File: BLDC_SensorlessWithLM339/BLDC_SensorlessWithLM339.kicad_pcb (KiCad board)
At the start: 2 copper layers, 98 x 98 mm, 48 parts, among them J1 Conn_01x04_Female, J2 Conn_01x07_Female, J3 Screw_Terminal_01x02, J4 Screw_Terminal_01x03, Q1 50N06, Q2 50N06, Q3 50N06, Q4 50N06, Q5 50N06, Q6 50N06, U1 IR2101, U2 IR2101, U3 IR2101, U4 LM339N

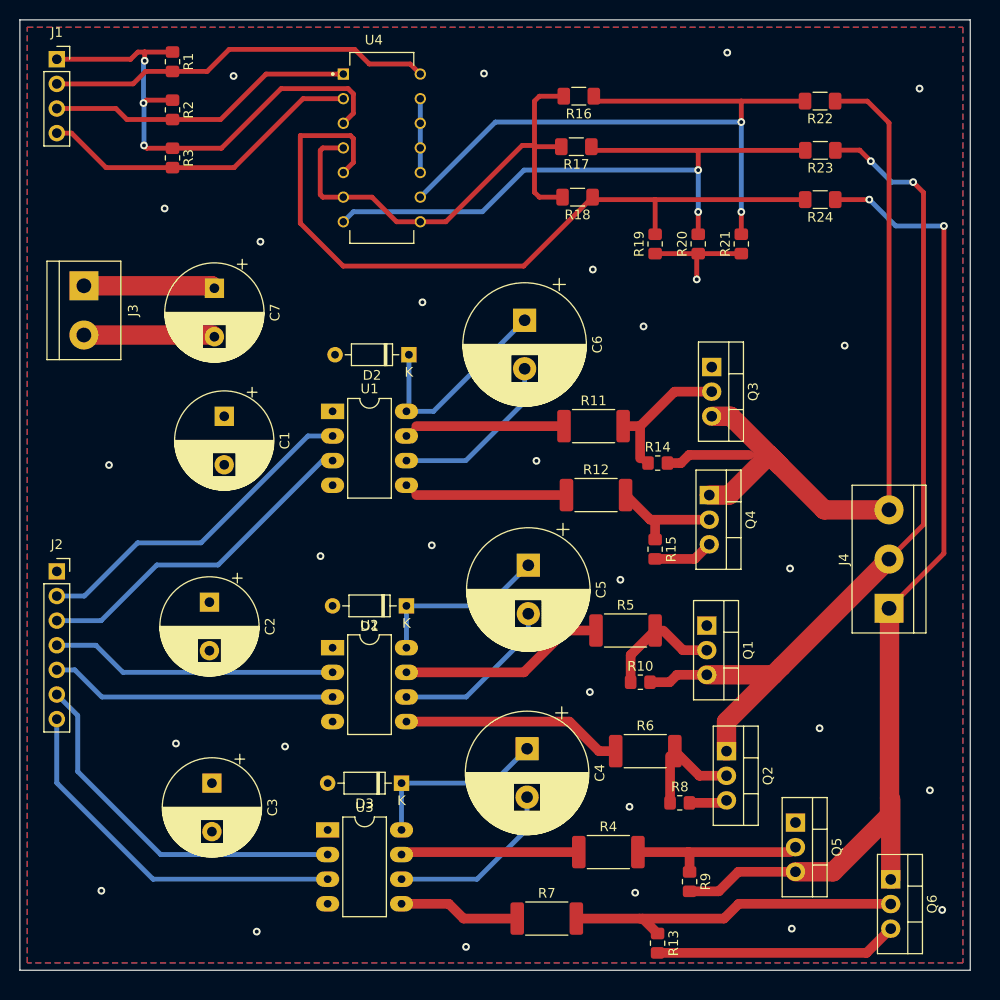
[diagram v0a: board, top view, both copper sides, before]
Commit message: Version 0.3
I ordered the PCB. I will test it when it arrives.
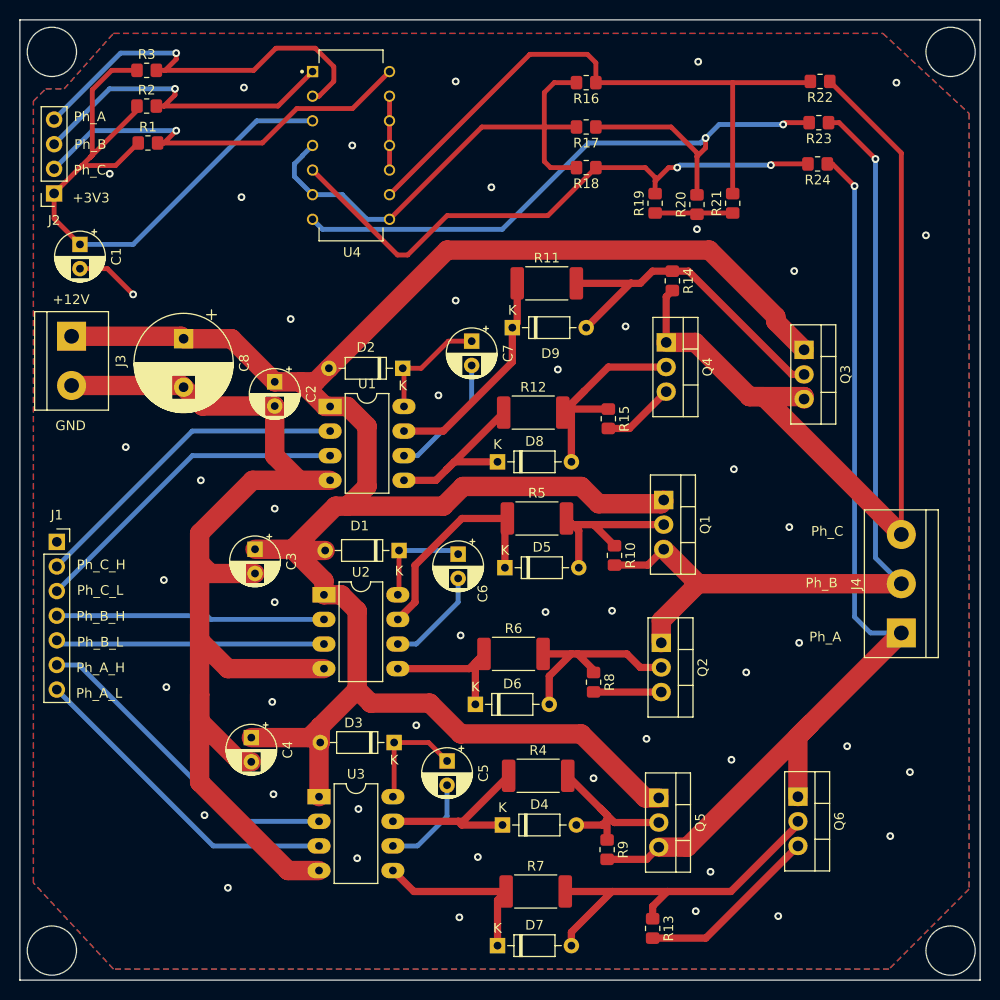
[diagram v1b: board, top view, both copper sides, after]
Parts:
- added C8: 470u, Capacitor_THT:CP_Radial_D10.0mm_P5.00mm, F.Cu at (28.8, 44.8)
- added D4: 1N4148, Diode_THT:D_DO-35_SOD27_P7.62mm_Horizontal, F.Cu at (61.7, 95.0)
- added D5: 1N4148, Diode_THT:D_DO-35_SOD27_P7.62mm_Horizontal, F.Cu at (62.0, 68.5)
- added D6: 1N4148, Diode_THT:D_DO-35_SOD27_P7.62mm_Horizontal, F.Cu at (58.9, 82.5)
- added D7: 1N4148, Diode_THT:D_DO-35_SOD27_P7.62mm_Horizontal, F.Cu at (61.2, 107.4)
- added D8: 1N4148, Diode_THT:D_DO-35_SOD27_P7.62mm_Horizontal, F.Cu at (61.2, 57.5)
- added D9: 1N4148, Diode_THT:D_DO-35_SOD27_P7.62mm_Horizontal, F.Cu at (62.7, 43.7)
- C1, C2, C3: footprint Capacitor_THT:CP_Radial_D10.0mm_P5.00mm -> Capacitor_THT:CP_Radial_D5.0mm_P2.50mm
- C4: value 2u2 -> 10u; footprint Capacitor_THT:CP_Radial_D12.5mm_P5.00mm -> Capacitor_THT:CP_Radial_D5.0mm_P2.50mm
- C5, C6: footprint Capacitor_THT:CP_Radial_D12.5mm_P5.00mm -> Capacitor_THT:CP_Radial_D5.0mm_P2.50mm
- C7: value 470u -> 2u2; footprint Capacitor_THT:CP_Radial_D10.0mm_P5.00mm -> Capacitor_THT:CP_Radial_D5.0mm_P2.50mm
- J1: value Conn_01x04_Female -> Conn_01x07_Female; footprint Connector_PinSocket_2.54mm:PinSocket_1x04_P2.54mm_Vertical -> Connector_PinSocket_2.54mm:PinSocket_1x07_P2.54mm_Vertical
- J2: value Conn_01x07_Female -> Conn_01x04_Female; footprint Connector_PinSocket_2.54mm:PinSocket_1x07_P2.54mm_Vertical -> Connector_PinSocket_2.54mm:PinSocket_1x04_P2.54mm_Vertical
- R10, R13, R14, R15, R8, R9: value 220 -> 10k
- R11, R12, R4, R5, R6, R7: value 10_2W -> 10_1W
- R16, R17, R18, R22, R23, R24: footprint Resistor_SMD:R_1206_3216Metric_Pad1.30x1.75mm_HandSolder -> Resistor_SMD:R_0805_2012Metric_Pad1.20x1.40mm_HandSolder
- moved J1 49.8 mm to (15.7, 65.8)
- moved J2 39.0 mm to (15.5, 29.8), turned to 180 degrees
- moved C4 28.5 mm to (35.8, 86.0)
- moved C7 27.1 mm to (58.5, 45.1)
- moved C6 25.1 mm to (57.1, 67.1)
- moved C3 24.5 mm to (36.2, 66.5)
- moved C2 23.7 mm to (38.2, 49.3)
- moved C1 23.1 mm to (18.1, 35.1)
- moved C5 21.9 mm to (56.0, 88.4)
- moved R14 18.9 mm to (79.2, 38.9), turned to 270 degrees
- moved R6 16.9 mm to (62.9, 77.3)
- moved Q4 16.4 mm to (78.6, 45.2)
- moved R11 15.5 mm to (66.3, 39.1)
- moved R8 15.3 mm to (71.1, 80.3), turned to 270 degrees
- moved R5 14.7 mm to (65.3, 63.4)
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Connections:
- C1 pad 1: +12V -> +3V3
- C4 pad 1: Net-(C4-Pad1) -> +12V
- C4 pad 2: Net-(C4-Pad2) -> GND
- C7 pad 1: +12V -> Net-(C7-Pad1)
- C7 pad 2: GND -> Net-(C7-Pad2)
- D1 pad 1: Net-(C5-Pad1) -> Net-(C6-Pad1)
- D2 pad 1: Net-(C6-Pad1) -> Net-(C7-Pad1)
- D3 pad 1: Net-(C4-Pad1) -> Net-(C5-Pad1)
- J1 pad 1: +3V3 -> Net-(J1-Pad1)
- J2 pad 1: Net-(J2-Pad1) -> +3V3
- R1 pad 2: Net-(J1-Pad2) -> Net-(J2-Pad2)
- R2 pad 2: Net-(J1-Pad3) -> Net-(J2-Pad3)
- R3 pad 2: Net-(J1-Pad4) -> Net-(J2-Pad4)
- U1 pad 2: Net-(J2-Pad2) -> Net-(J1-Pad2)
- U1 pad 3: Net-(J2-Pad3) -> Net-(J1-Pad3)
- U1 pad 6: Net-(C6-Pad2) -> Net-(C7-Pad2)
- U1 pad 8: Net-(C6-Pad1) -> Net-(C7-Pad1)
- U2 pad 2: Net-(J2-Pad4) -> Net-(J1-Pad4)
- U2 pad 3: Net-(J2-Pad5) -> Net-(J1-Pad5)
- U2 pad 6: Net-(C5-Pad2) -> Net-(C6-Pad2)
- U2 pad 8: Net-(C5-Pad1) -> Net-(C6-Pad1)
- U3 pad 2: Net-(J2-Pad6) -> Net-(J1-Pad6)
- U3 pad 3: Net-(J2-Pad7) -> Net-(J1-Pad7)
- U3 pad 6: Net-(C4-Pad2) -> Net-(C5-Pad2)
- U3 pad 8: Net-(C4-Pad1) -> Net-(C5-Pad1)
- U4 pad 1: Net-(J1-Pad3) -> Net-(J2-Pad3)
- U4 pad 14: Net-(J1-Pad2) -> Net-(J2-Pad2)
- U4 pad 2: Net-(J1-Pad4) -> Net-(J2-Pad4)
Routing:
- net +12V: track 13.6 -> 228.9 mm
- net GND: track 68.0 -> 173.8 mm, vias 29 -> 48
- net Net-(J2-Pad7): track 38.6 -> 0.00 mm
- net Net-(J2-Pad6): track 38.2 -> 0.00 mm
- net Net-(J1-Pad7): track 0.00 -> 33.7 mm
- net Net-(J1-Pad6): track 0.00 -> 33.7 mm
- net Net-(J2-Pad5): track 29.6 -> 0.00 mm
- net Net-(J1-Pad5): track 0.00 -> 27.7 mm
- net Net-(D9-Pad2): track 15.0 -> 35.0 mm
- net Net-(C4-Pad1): track 19.3 -> 0.00 mm
- net Net-(C4-Pad2): track 18.4 -> 0.00 mm
- net Net-(R18-Pad1): track 79.1 -> 61.3 mm, vias 0 -> 2
- net +3V3: track 53.0 -> 67.9 mm, vias 3 -> 0
- net Net-(D8-Pad2): track 12.0 -> 25.3 mm
- net Net-(C7-Pad2): track 0.00 -> 13.0 mm
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- added copper zone on F.Cu, net GND
- removed copper zone on F.Cu, net +12V
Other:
- board size 98 x 98 mm -> 99.1 x 99.1 mm
- net class PWR_12V: clearance 0.5 -> 0.2; via_dia 1.6 -> 0.8; via_drill 1 -> 0.4
- board text added: "+12V"
- board text added: "+3V3"
- board text added: "GND"
- board text added: "Ph_A"
- board text added: "Ph_A_H"
- board text added: "Ph_A_L"
- board text added: "Ph_B"
- board text added: "Ph_B_H"
- board text added: "Ph_B_L"
- board text added: "Ph_C"
- board text added: "Ph_C_H"
- board text added: "Ph_C_L"
